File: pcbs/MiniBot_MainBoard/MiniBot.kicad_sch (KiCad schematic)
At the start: 40 parts, among them IC1 MMC5633NJL, IC2 MIC23050-SYML-TR, J1 Conn_01x08, J2 Conn_01x02, J3 GSB1C41110SSHR, U1 ESP32-C3-MINI-1-H4X, U3 MCP73832-2-OT

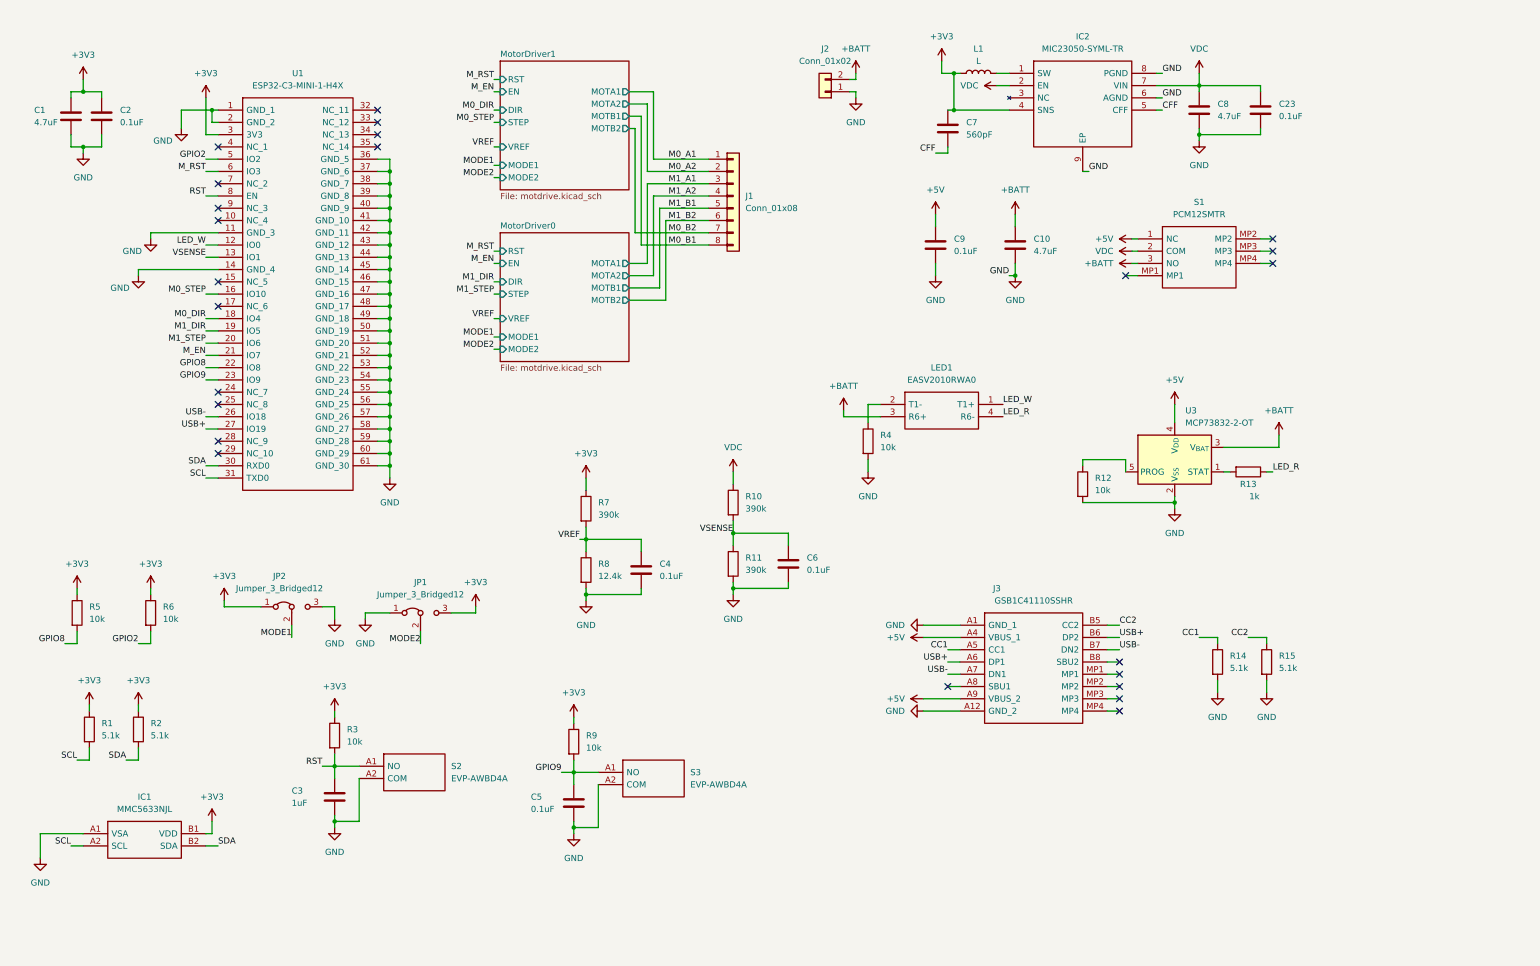
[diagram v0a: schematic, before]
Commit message: cleanup minibot schematic
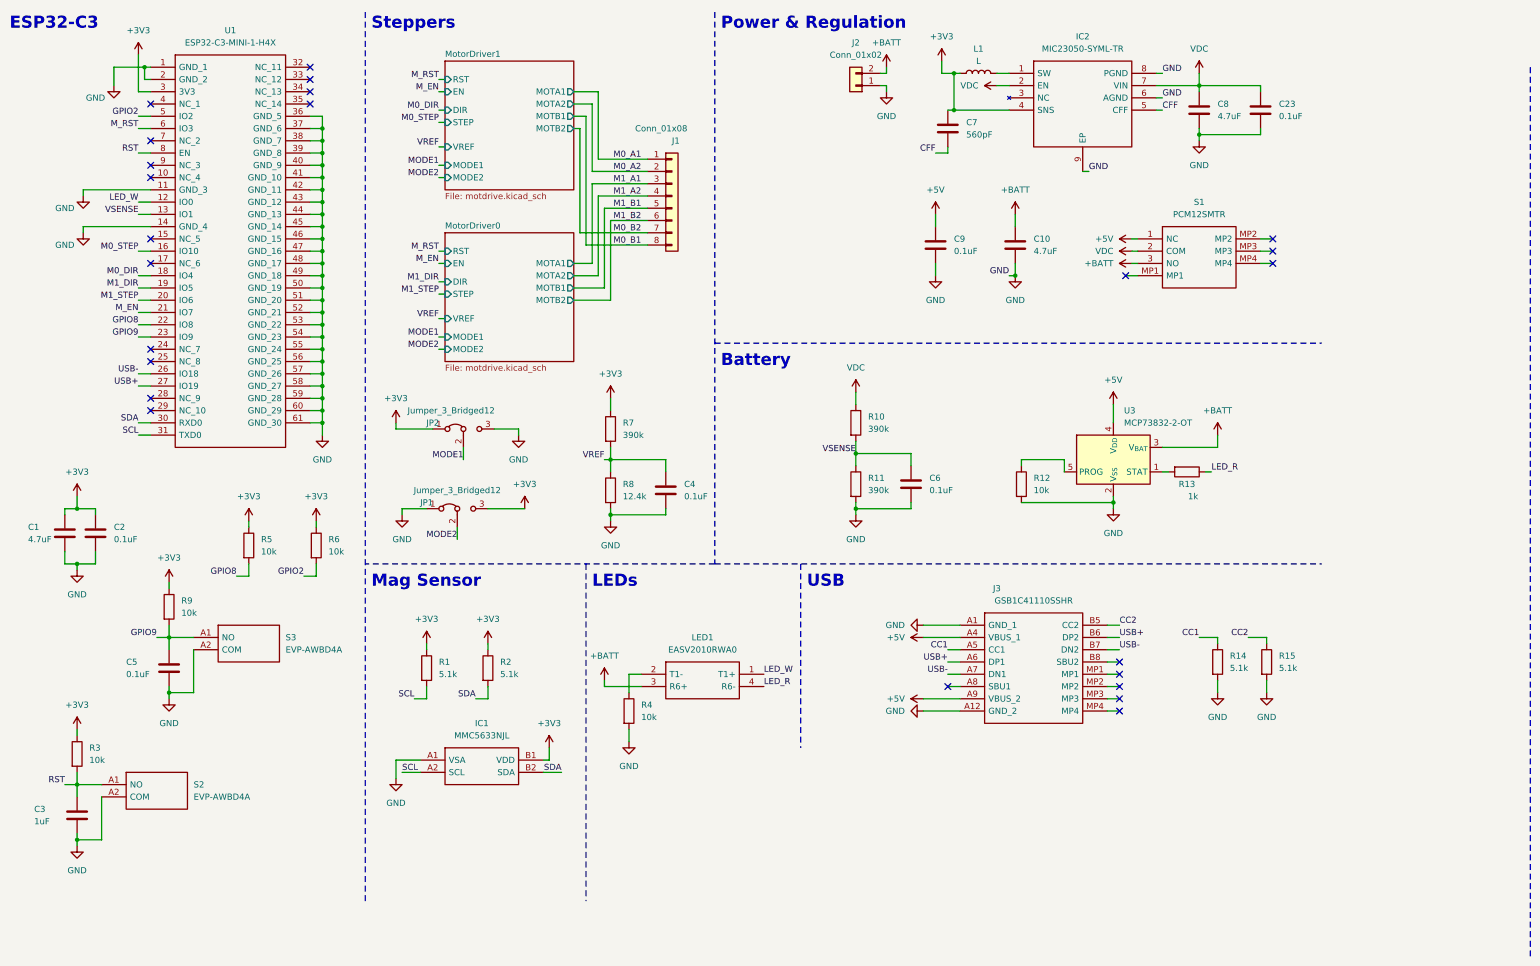
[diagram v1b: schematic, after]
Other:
- note added: "Battery"
- note added: "ESP32-C3"
- note added: "LEDs"
- note added: "Mag Sensor"
- note added: "Power & Regulation"
- note added: "Steppers"
- note added: "USB"
- moved on the sheet: C1, C2, C3, C4, C5, C6, IC1, J1, J2, JP1, JP2, LED1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
